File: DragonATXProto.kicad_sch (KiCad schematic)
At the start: 26 parts, among them J5 Joystick ports, J6 MD-40SM

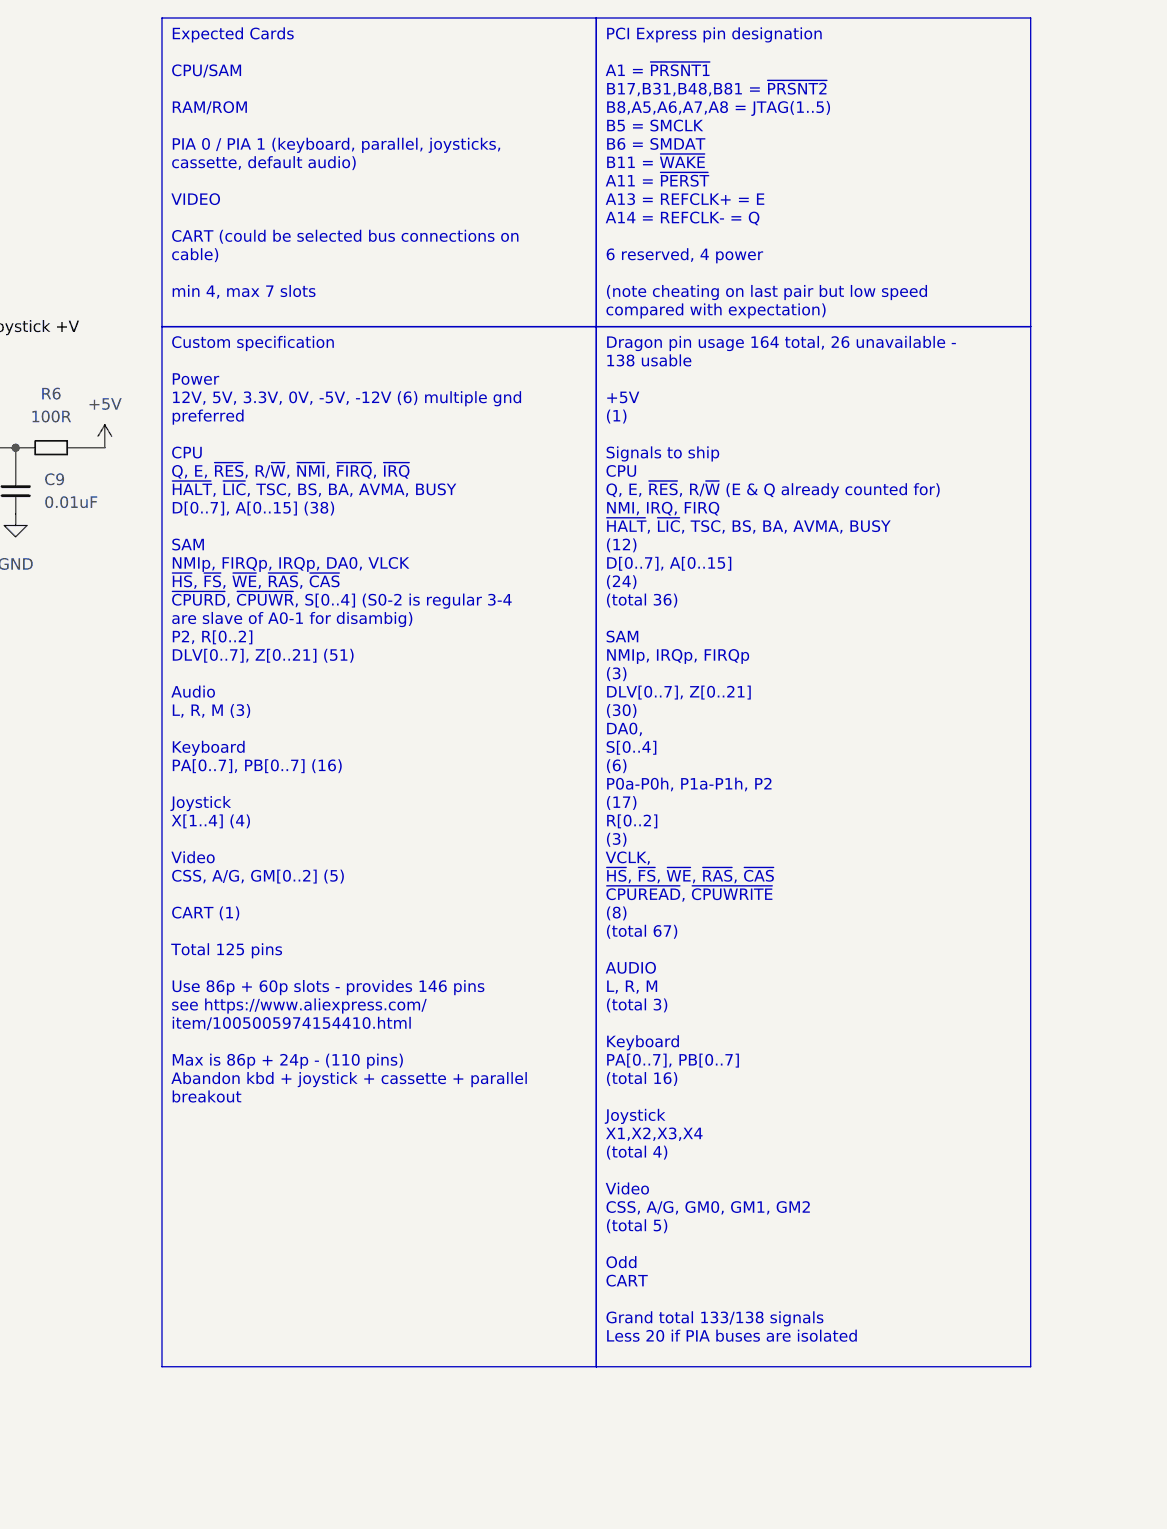
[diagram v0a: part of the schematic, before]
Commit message: add notes
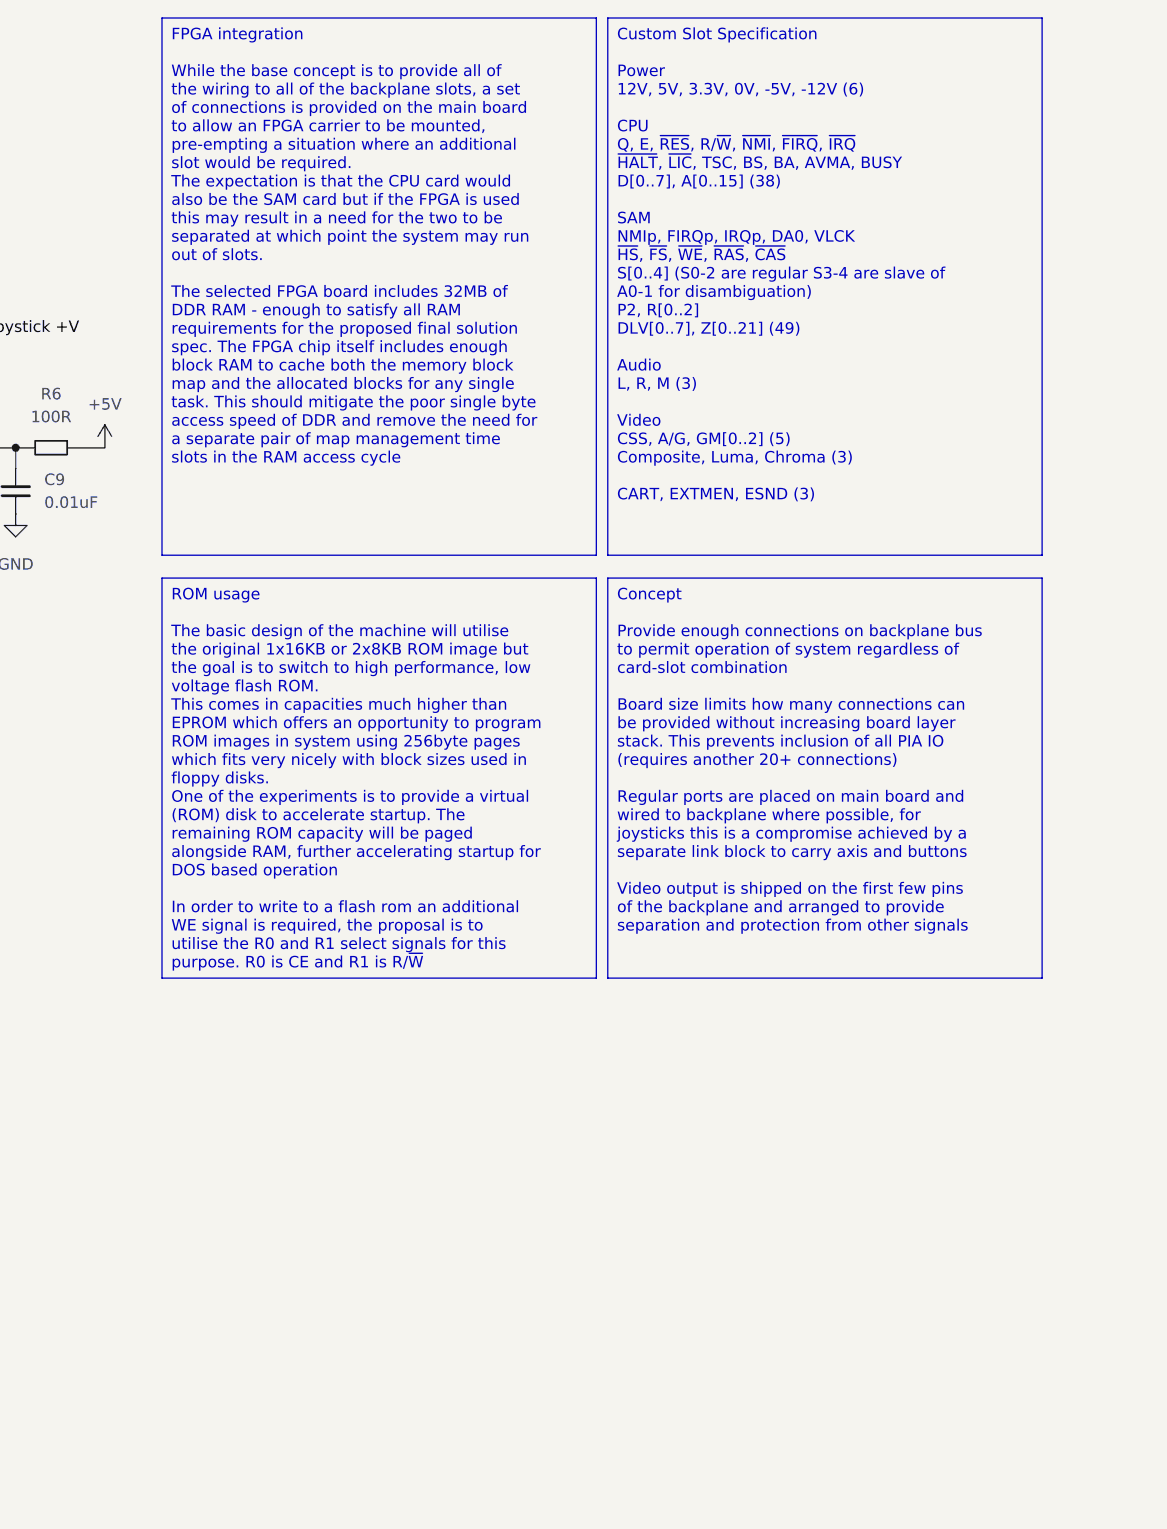
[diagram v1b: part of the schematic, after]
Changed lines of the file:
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@@
 		)
 	)
-	(text_box "Dragon pin usage 164 total, 26 unavailable - 138 usable\n\n+5V\n(1)\n\nSignals to ship\nCPU\nQ, E, ~{RES}, R/~{W} (E & Q already counted for)\nNMI, IRQ, FIRQ \n~{HALT}, ~{LIC}, TSC, BS, BA, AVMA, BUSY\n(12)\nD[0..7], A[0..15]\n(24)\n(total 36)\n\nSAM\nNMIp, IRQp, FIRQp\n(3)\nDLV[0..7], Z[0..21]\n(30)\nDA0,\nS[0..4]\n(6)\nP0a-P0h, P1a-P1h, P2\n(17)\nR[0..2]\n(3)\nVCLK,\n~{HS}, ~{FS}, ~{WE}, ~{RAS}, ~{CAS}\n~{CPUREAD}, ~{CPUWRITE}\n(8)\n(total 67)\n\nAUDIO\nL, R, M\n(total 3)\n\nKeyboard\nPA[0..7], PB[0..7]\n(total 16)\n\nJoystick\nX1,X2,X3,X4\n(total 4)\n\nVideo\nCSS, A/G, GM0, GM1, GM2\n(total 5)\n\nOdd\nCART\n\nGrand total 133/138 signals\nLess 20 if PIA buses are isolated"
+	(text_box "ROM usage\n\nThe basic design of the machine will utilise the original 1x16KB or 2x8KB ROM image but the goal is to switch to high performance, low voltage flash ROM. \nThis comes in capacities much higher than EPROM which offers an opportunity to program ROM images in system using 256byte pages which fits very nicely with block sizes used in floppy disks.\nOne of the experiments is to provide a virtual (ROM) disk to accelerate startup. The remaining ROM capacity will be paged alongside RAM, further accelerating startup for DOS based operation\n\nIn order to write to a flash rom an additional WE signal is required, the proposal is to utilise the R0 and R1 select signals for this purpose. R0 is CE and R1 is R/~{W}"
 		(exclude_from_sim no)
-		(at 233.68 48.26 0)
-		(size 48.26 115.57)
-		(stroke
-			(width 0)
-			(type default)
-		)
-		(fill
-			(type color)
-			(color 185 255 112 1)
-		)
-		(effects
-			(font
-				(size 1.27 1.27)
-			)
-			(justify left top)
-		)
-	)
-	(text_box "Expected Cards\n\nCPU/SAM\n\nRAM/ROM\n\nPIA 0 / PIA 1 (keyboard, parallel, joysticks, cassette, default audio)\n\nVIDEO\n\nCART (could be selected bus connections on cable)\n\nmin 4, max 7 slots"
-		(exclude_from_sim no)
-		(at 185.42 13.97 0)
-		(size 48.26 34.29)
-		(stroke
-			(width 0)
-			(type default)
-		)
-		(fill
-			(type color)
-			(color 255 249 138 1)
-		)
-		(effects
-			(font
-				(size 1.27 1.27)
-			)
-			(justify left top)
-		)
-	)
-	(text_box "Custom specification\n\nPower\n12V, 5V, 3.3V, 0V, -5V, -12V (6) multiple gnd preferred\n\nCPU\nQ, E, ~{RES}, R/~{W}, ~{NMI}, ~{FIRQ}, ~{IRQ}\n~{HALT}, ~{LIC}, TSC, BS, BA, AVMA, BUSY\nD[0..7], A[0..15] (38)\n\nSAM\nNMIp, FIRQp, IRQp, DA0, VLCK\n~{HS}, ~{FS}, ~{WE}, ~{RAS}, ~{CAS}\n~{CPURD}, ~{CPUWR}, S[0..4] (S0-2 is regular 3-4 are slave of A0-1 for disambig)\nP2, R[0..2] \nDLV[0..7], Z[0..21] (51)\n\nAudio\nL, R, M (3)\n\nKeyboard\nPA[0..7], PB[0..7] (16)\n\nJoystick\nX[1..4] (4)\n\nVideo\nCSS, A/G, GM[0..2] (5)\n\nCART (1)\n\nTotal 125 pins\n\nUse 86p + 60p slots - provides 146 pins\nsee https://www.aliexpress.com/\nitem/1005005974154410.html\n\nMax is 86p + 24p - (110 pins)\nAbandon kbd + joystick + cassette + parallel breakout"
-		(exclude_from_sim no)
-		(at 185.42 48.26 0)
-		(size 48.26 115.57)
+		(at 185.42 76.2 0)
+		(size 48.26 44.45)
 		(stroke
 			(width 0)
@@
 		)
 	)
-	(text_box "PCI Express pin designation\n\nA1 = ~{PRSNT1}\nB17,B31,B48,B81 = ~{PRSNT2}\nB8,A5,A6,A7,A8 = JTAG(1..5)\nB5 = SMCLK\nB6 = SMDAT\nB11 = ~{WAKE}\nA11 = ~{PERST}\nA13 = REFCLK+ = E\nA14 = REFCLK- = Q\n\n6 reserved, 4 power\n\n(note cheating on last pair but low speed compared with expectation)"
+	(text_box "FPGA integration\n\nWhile the base concept is to provide all of the wiring to all of the backplane slots, a set of connections is provided on the main board to allow an FPGA carrier to be mounted, pre-empting a situation where an additional slot would be required.\nThe expectation is that the CPU card would also be the SAM card but if the FPGA is used this may result in a need for the two to be separated at which point the system may run out of slots.\n\nThe selected FPGA board includes 32MB of DDR RAM - enough to satisfy all RAM requirements for the proposed final solution spec. The FPGA chip itself includes enough block RAM to cache both the memory block map and the allocated blocks for any single task. This should mitigate the poor single byte access speed of DDR and remove the need for a separate pair of map management time slots in the RAM access cycle"
 		(exclude_from_sim no)
-		(at 233.68 13.97 0)
-		(size 48.26 34.29)
+		(at 185.42 13.97 0)
+		(size 48.26 59.69)
 		(stroke
 			(width 0)
+			(type default)
+		)
+		(fill
+			(type none)
+		)
+		(effects
+			(font
+				(size 1.27 1.27)
+			)
+			(justify left top)
+		)
+	)
+	(text_box "Custom Slot Specification\n\nPower\n12V, 5V, 3.3V, 0V, -5V, -12V (6)\n\nCPU\nQ, E, ~{RES}, R/~{W}, ~{NMI}, ~{FIRQ}, ~{IRQ}\n~{HALT}, ~{LIC}, TSC, BS, BA, AVMA, BUSY\nD[0..7], A[0..15] (38)\n\nSAM\nNMIp, FIRQp, IRQp, DA0, VLCK\n~{HS}, ~{FS}, ~{WE}, ~{RAS}, ~{CAS}\nS[0..4] (S0-2 are regular S3-4 are slave of A0-1 for disambiguation)\nP2, R[0..2] \nDLV[0..7], Z[0..21] (49)\n\nAudio\nL, R, M (3)\n\nVideo\nCSS, A/G, GM[0..2] (5)\nComposite, Luma, Chroma (3)\n\nCART, EXTMEN, ESND (3)"
+		(exclude_from_sim no)
+		(at 234.95 13.97 0)
+		(size 48.26 59.69)
+		(stroke
+			(width 0)
+			(type default)
+		)
+		(fill
+			(type none)
+		)
+		(effects
+			(font
+				(size 1.27 1.27)
+			)
+			(justify left top)
+		)
+	)
+	(text_box "Concept\n\nProvide enough connections on backplane bus to permit operation of system regardless of card-slot combination\n\nBoard size limits how many connections can be provided without increasing board layer stack. This prevents inclusion of all PIA IO (requires another 20+ connections)\n\nRegular ports are placed on main board and wired to backplane where possible, for joysticks this is a compromise achieved by a separate link block to carry axis and buttons\n\nVideo output is shipped on the first few pins of the backplane and arranged to provide separation and protection from other signals"
+		(exclude_from_sim no)
+		(at 234.95 76.2 0)
+		(size 48.26 44.45)
+		(stroke
+			(width 0)

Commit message: revise bus tracing
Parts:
- RL1: DigiKey (none) -> PB1623-ND
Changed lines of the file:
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@@
 			)
 		)
-		(property "Datasheet" ""
+		(property "Datasheet" "https://www.te.com/commerce/DocumentDelivery/DDEController?Action=srchrtrv&DocNm=108-98010&DocType=Specification%20Or%20Standard&DocLang=English&DocFormat=pdf&PartCntxt=3-1393779-3"
 			(at 57.15 85.598 0)
 			(effects
@@
 			(at 57.15 85.598 0)
 			(effects
+				(font
+					(size 1.27 1.27)
+				)
+				(hide yes)
+			)
+		)
+		(property "DigiKey" "PB1623-ND"
+			(at 57.15 85.598 0)
+			(effects
